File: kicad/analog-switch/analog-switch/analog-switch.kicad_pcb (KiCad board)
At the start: 2 copper layers, 17.8 x 43.2 mm, 11 parts, among them J1 Conn_01x04, J2 Conn_01x16_MountingPin, J4 Conn_01x04, J5 Conn_01x16_MountingPin, Q1 Q_PNP_EBC, U1 CD74HC4067M, U2 74HC595, U3 CD74HC4067M

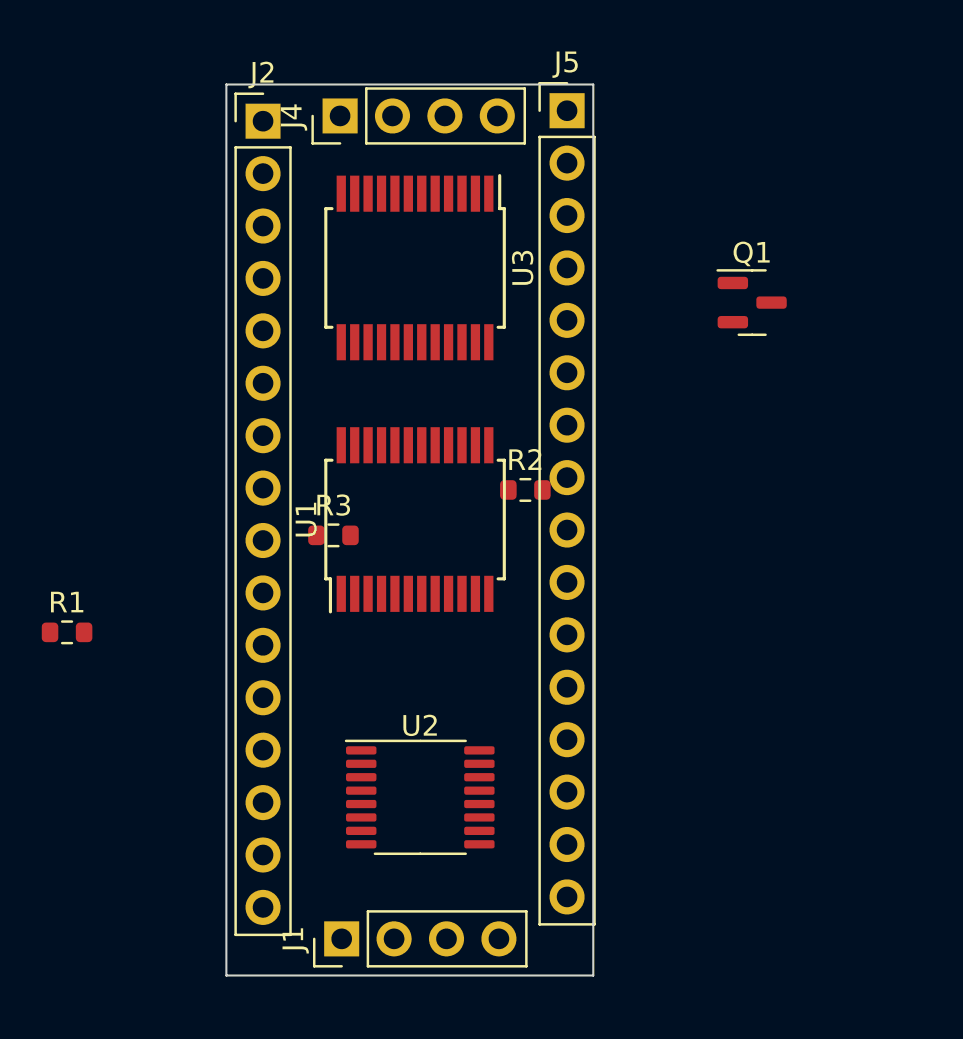
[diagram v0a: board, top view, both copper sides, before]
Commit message: proj settings
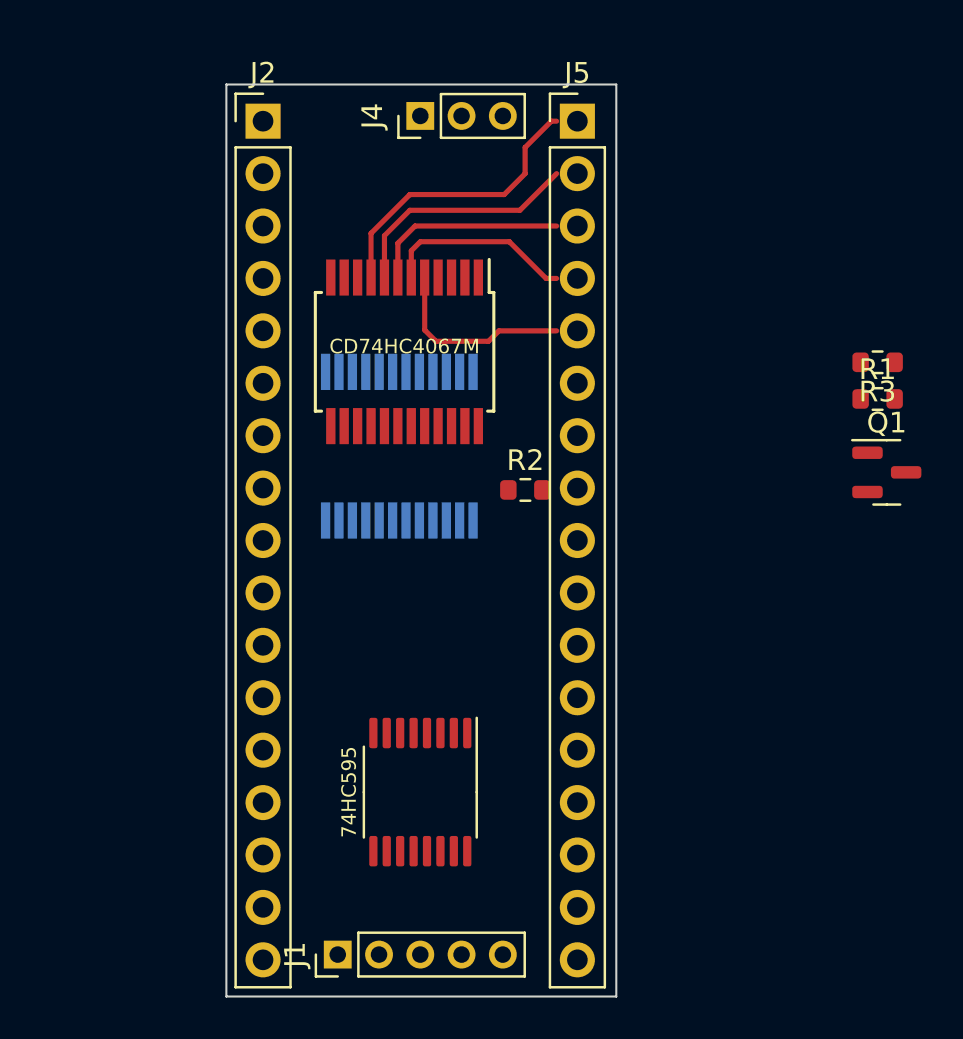
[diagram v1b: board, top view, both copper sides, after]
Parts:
- J1: value Conn_01x04 -> Conn_01x05_Male; footprint Connector_PinHeader_2.54mm:PinHeader_1x04_P2.54mm_Vertical -> Connector_PinHeader_2.00mm:PinHeader_1x05_P2.00mm_Vertical
- J2, J5: value Conn_01x16_MountingPin -> Conn_01x17_Male; footprint Connector_PinHeader_2.54mm:PinHeader_1x16_P2.54mm_Vertical -> Connector_PinHeader_2.54mm:PinHeader_1x17_P2.54mm_Vertical
- J4: value Conn_01x04 -> Conn_01x03_Female; footprint Connector_PinHeader_2.54mm:PinHeader_1x04_P2.54mm_Vertical -> Connector_PinHeader_2.00mm:PinHeader_1x03_P2.00mm_Vertical
- U1: moved to B.Cu
- moved R1 40.9 mm to (82.4, 66.0)
- moved R3 27.7 mm to (82.4, 64.3), turned to 180 degrees
- moved Q1 10.5 mm to (82.8, 69.6)
- moved U3 4.10 mm to (59.4, 63.8)
- moved J4 3.89 mm to (60.2, 52.3)
- moved U1 3.64 mm to (59.2, 68.3), turned to -90 degrees
- moved J1 0.79 mm to (56.2, 93.0)
- moved J5 0.71 mm to (67.8, 52.6)
- moved U2 0.25 mm to (60.2, 85.1), turned to -90 degrees
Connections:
- J1 pad 1: Net-(J1-Pad1) -> AN1
- J1 pad 2: Net-(J1-Pad2) -> AN2
- J1 pad 4: GND -> Net-(J1-Pad4)
- J4 pad 3: Net-(J1-Pad3) -> Net-(J1-Pad5)
- R1 pad 2: Net-(J1-Pad3) -> Net-(J1-Pad5)
- R2 pad 1: Net-(J1-Pad3) -> Net-(Q1-Pad2)
- R2 pad 2: Net-(Q1-Pad2) -> Net-(J1-Pad5)
- R3 pad 1: Net-(Q1-Pad3) -> GND
- R3 pad 2: GND -> Net-(Q1-Pad3)
- U1 pad 1: Net-(J3-Pada1) -> AN1
- U2 pad 11: Net-(J1-Pad2) -> Net-(J1-Pad4)
- U2 pad 13: Net-(J1-Pad3) -> Net-(J1-Pad5)
- U2 pad 14: Net-(J1-Pad1) -> Net-(J1-Pad3)
- U3 pad 1: Net-(J3-Padb1) -> AN2
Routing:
- net Net-(J5-Pad1): track 0.00 -> 14.1 mm
- net Net-(J5-Pad2): track 0.00 -> 11.6 mm
- net Net-(J5-Pad3): track 0.00 -> 9.70 mm
- net Net-(J5-Pad5): track 0.00 -> 9.37 mm
- net Net-(J5-Pad4): track 0.00 -> 9.26 mm
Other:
- board size 17.8 x 43.2 mm -> 18.9 x 44.2 mm
